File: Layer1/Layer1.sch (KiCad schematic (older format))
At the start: 48 parts, among them IC1 74HCT4060D-Q100,11, J1 Conn_02x20_Odd_Even, J2 Conn_02x20_Odd_Even, J3 Conn_02x12_Odd_Even, J4 Barrel_Jack_MountingPin, Q1 2N2222, SW1 SW_Push, SW2 SW_Push, SW3 SW_DIP_x01, U1 28C256, U10 7400, U11 NE555, U2 74LS193, U3 74461, U4 28C256, U5 74154, U6 74461, U7 28C256, U8 74HCT273, U9 28C256, X1 SG-8002DC

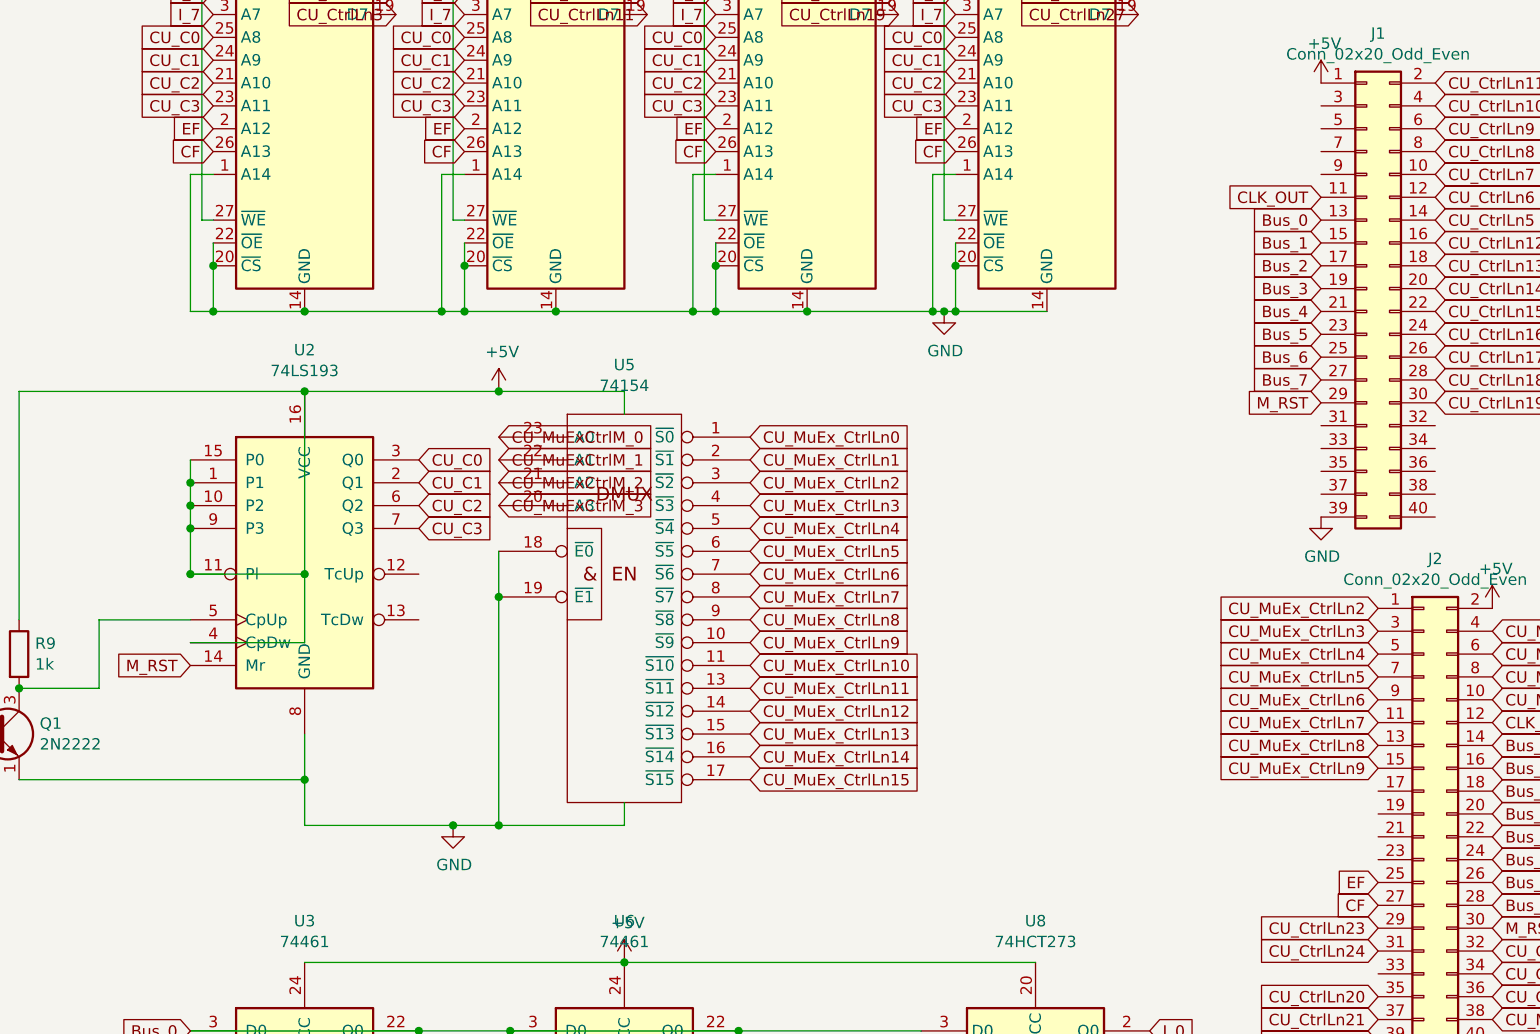
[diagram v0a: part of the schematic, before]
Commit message: Layer 3 complete
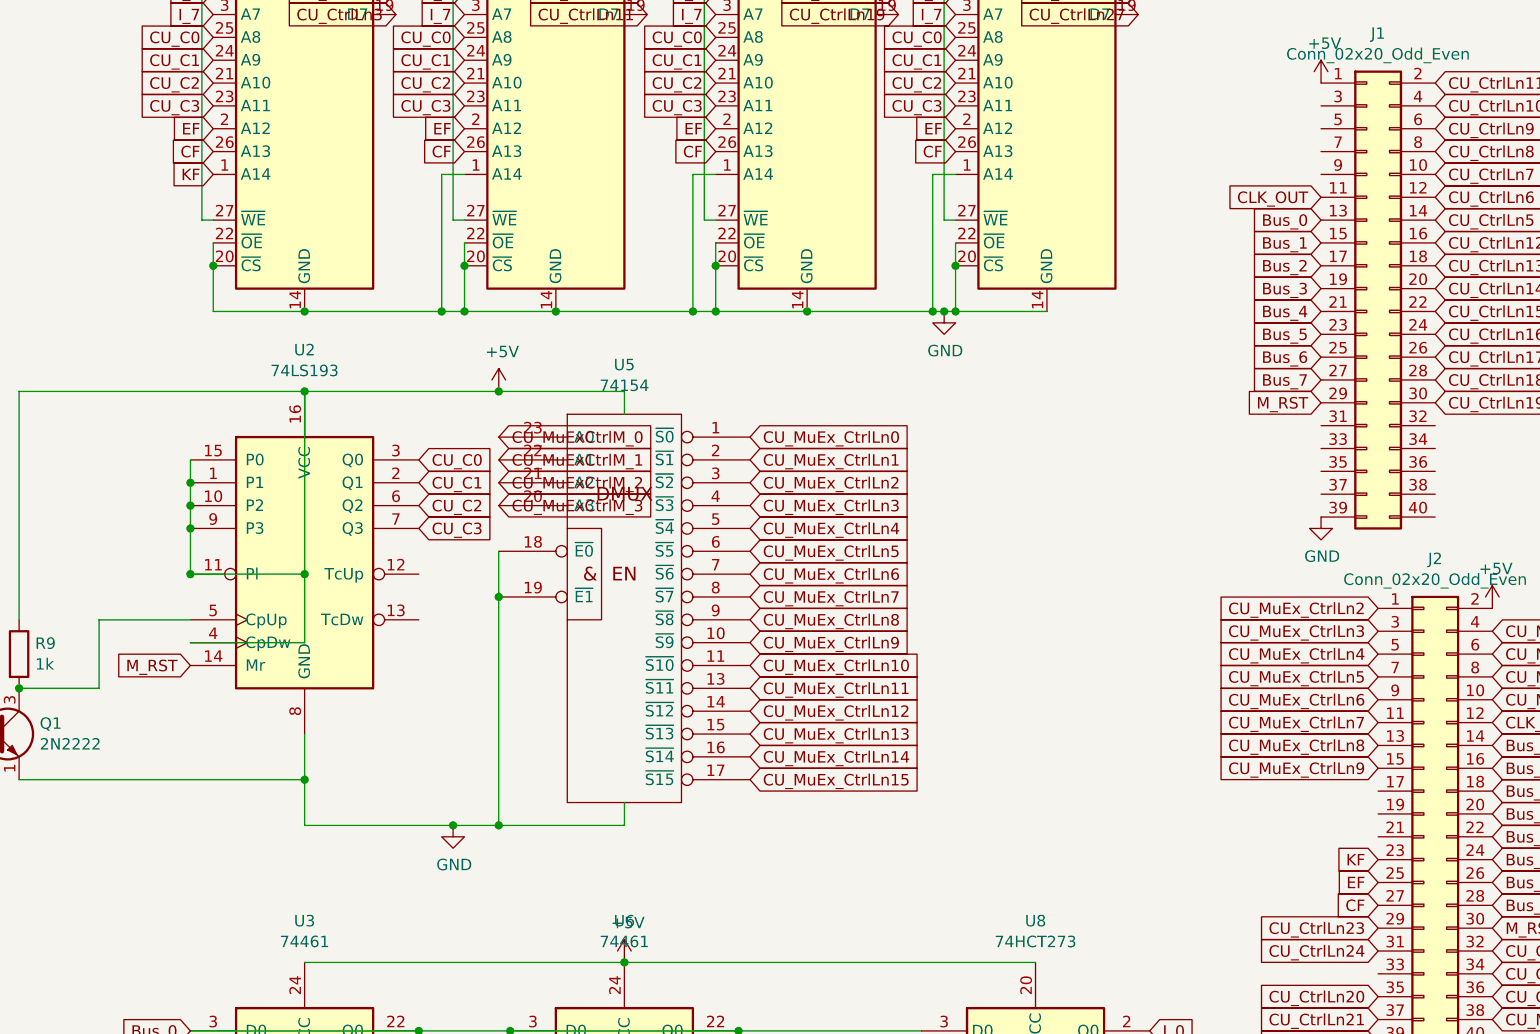
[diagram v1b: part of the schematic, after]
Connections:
- net GND: no longer U1.1 (A14)
- net KF: now reaches J2.23 (Pin_23)
- net KF: now also U1.1 (A14)
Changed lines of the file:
@@
 EESchema Schematic File Version 4
+LIBS:Layer1-cache
 EELAYER 30 0
 EELAYER END
@@
 Connection ~ 2500 2950
 Connection ~ 3600 2950
-Wire Wire Line
-	3600 2950 4150 2950
-Wire Wire Line
-	2500 2950 3100 2950
-Wire Wire Line
-	2100 2950 2000 2950
 Connection ~ 2100 2950
 Connection ~ 1400 2950
@@
 Text GLabel 4250 2250 0    50   Input ~ 0
 CF
-Wire Wire Line
-	1000 2350 900  2350
-Wire Wire Line
-	900  2350 900  2950
-Wire Wire Line
-	900  2950 1000 2950
-Connection ~ 1000 2950
-Wire Wire Line
-	2100 2350 2000 2350
-Wire Wire Line
-	2000 2350 2000 2950
-Connection ~ 2000 2950
-Wire Wire Line
-	2000 2950 1400 2950
-Wire Wire Line
-	3200 2350 3100 2350
-Wire Wire Line
-	3100 2350 3100 2950
-Connection ~ 3100 2950
-Wire Wire Line
-	3100 2950 3200 2950
-Wire Wire Line
-	4250 2350 4150 2350
-Wire Wire Line
-	4150 2350 4150 2950
-Connection ~ 4150 2950
-Wire Wire Line
-	4150 2950 4200 2950
 $Comp
 L Connector_Generic:Conn_02x20_Odd_Even J1
@@
 Text GLabel 6100 5550 0    50   Input ~ 0
 CF
+Wire Wire Line
+	1400 2950 2000 2950
+Wire Wire Line
+	2500 2950 3100 2950
+Wire Wire Line
+	3600 2950 4150 2950
+Text GLabel 1000 2350 0    50   Input ~ 0
+KF
+Text GLabel 6100 5350 0    50   Input ~ 0
+KF
+Wire Wire Line
+	2100 2350 2000 2350
+Wire Wire Line
+	2000 2350 2000 2950
+Connection ~ 2000 2950
+Wire Wire Line
+	2000 2950 2100 2950
+Wire Wire Line
+	3200 2350 3100 2350
+Wire Wire Line
+	3100 2350 3100 2950
+Connection ~ 3100 2950
+Wire Wire Line
+	3100 2950 3200 2950
+Wire Wire Line
+	4250 2350 4150 2350
+Wire Wire Line
+	4150 2350 4150 2950
+Connection ~ 4150 2950
+Wire Wire Line
+	4150 2950 4200 2950
 $EndSCHEMATC

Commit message: Backup
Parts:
- removed Q1: 2N2222, Package_TO_SOT_THT:TO-92, symbol Transistor_BJT:2N2219
- removed R8: 10k, Resistor_THT:R_Axial_DIN0309_L9.0mm_D3.2mm_P12.70mm_Horizontal, symbol Device:R
- removed R9: 1k, Resistor_THT:R_Axial_DIN0309_L9.0mm_D3.2mm_P12.70mm_Horizontal, symbol Device:R
- removed U10: 7400, Package_DIP:DIP-14_W7.62mm, symbol 74xx:7400
- added U10, U18: 74LS08, Package_DIP:DIP-14_W7.62mm_LongPads, symbol 74xx:74LS08
- added U12, U16, U20: 74LS04, Package_DIP:DIP-14_W7.62mm_LongPads, symbol 74xx:74LS04
- added U13, U15, U17: 74LS02, Package_DIP:DIP-14_W7.62mm_LongPads, symbol 74xx:74LS02
- added U14, U19: 74LS00, Package_DIP:DIP-14_W7.62mm_LongPads, symbol 74xx:74LS00
- added U21: SST39SF010, Package_DIP:DIP-32_W15.24mm_LongPads, symbol Memory_Flash:SST39SF010
- added U22: 74HC238, Package_DIP:DIP-16_W7.62mm_LongPads, symbol 74xx_IEEE:74HC238
- added U23: 74LS138, Package_DIP:DIP-16_W7.62mm_LongPads, symbol 74xx_IEEE:74LS138
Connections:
- net +5V: now also U10.14 (VCC), U12.14 (VCC), U13.14 (VCC), U14.14 (VCC), U15.14 (VCC), U16.14 (VCC), U17.14 (VCC), U19.14 (VCC), U20.14 (VCC), U21.32 (VCC), U22.16 (VCC), U23.16 (VCC), U23.6 (G1)
- net 555_OUT: now also U19.1
- net BTN_OUT: now also U19.5
- net CF: now also U21.28 (A13)
- net CLK_OUT: now also U16.11
- net CU_C0: now also J1.3 (Pin_3), U21.27 (A8)
- net CU_C1: now also J1.5 (Pin_5), U21.26 (A9)
- net CU_C2: now also J1.7 (Pin_7), U21.23 (A10)
- net CU_C3: now also J1.9 (Pin_9), U21.25 (A11)
- net CU_CtrlLn0: now also U10.12, U13.1
- net CU_CtrlLn1: now also U10.9, U14.8
- net CU_CtrlLn2: now also U10.4, U13.10
- net CU_CtrlLn27: now also U2.14 (Mr)
- net CU_CtrlLn3: now also U10.1, U14.3
- net CU_CtrlLn4: now also U15.2, U15.5, U17.3, U22.14 (Y1); no longer U8.11 (Cp)
- net CU_CtrlLn5: now also U15.3, U16.3, U17.8
- net CU_CtrlLn6: now also U15.6, U16.5
- net CU_MuEx_CtrlLn0: now also U5.3 (~S2); no longer U5.1 (~S0)
- net CU_MuEx_CtrlLn1: now also U5.4 (~S3); no longer U5.2 (~S1)
- net CU_MuEx_CtrlLn10: no longer U5.11 (~S10)
- net CU_MuEx_CtrlLn11: no longer U5.13 (~S11)
- net CU_MuEx_CtrlLn12: no longer U5.14 (~S12)
- net CU_MuEx_CtrlLn13: no longer U5.15 (~S13)
- net CU_MuEx_CtrlLn14: no longer U5.16 (~S14)
- net CU_MuEx_CtrlLn15: no longer U5.17 (~S15)
- net CU_MuEx_CtrlLn2: no longer U5.3 (~S2)
- net CU_MuEx_CtrlLn3: no longer U5.4 (~S3)
- net CU_MuEx_CtrlLn4: no longer U5.5 (~S4)
- net CU_MuEx_CtrlLn5: no longer U5.6 (~S5)
- net CU_MuEx_CtrlLn6: no longer U5.7 (~S6)
- net CU_MuEx_CtrlLn7: no longer U5.8 (~S7)
- net CU_MuEx_CtrlLn8: no longer U5.9 (~S8)
- net CU_MuEx_CtrlLn9: no longer U5.10 (~S9)
- net Debug_CLK_OUT: now also U19.8
- net EF: now also U21.4 (A12)
- net GND: now also U10.7 (GND), U12.7 (GND), U13.7 (GND), U14.7 (GND), U15.7 (GND), U16.7 (GND), U17.7 (GND), U19.7 (GND), U20.7 (GND), U21.16 (GND), U21.2 (A16), U21.22 (CE), U21.24 (OE), U22.5 (~G2B), U22.8 (GND), U23.8 (GND); no longer U4.1 (A14), U5.18 (~E0), U7.1 (A14), U9.1 (A14)
- net I_0: now also J1.31 (Pin_31), U21.12 (A0)
- net I_1: now also J1.33 (Pin_33), U21.11 (A1)
- net I_2: now also J1.35 (Pin_35), U21.10 (A2)
- net I_3: now also J1.37 (Pin_37), U21.9 (A3)
- net I_4: now also J1.32 (Pin_32), U21.8 (A4)
- net I_5: now also J1.34 (Pin_34), U21.7 (A5)
- net I_6: now also J1.36 (Pin_36), U18.12, U21.6 (A6); no longer U1.4 (A6)
- net I_7: now also J1.38 (Pin_38), U18.13, U21.5 (A7); no longer U1.3 (A7)
- net KF: now also U1.3 (A7), U21.29 (A14); no longer U1.1 (A14)
- net M_RST: now also U1.1 (A14), U4.1 (A14), U7.1 (A14), U9.1 (A14), U21.3 (A15); no longer U2.14 (Mr)
- net Switch_OUT: now also U16.9, U19.4
- net at U2.5 (CpUp): now also U16.10
- net CU_CtrlLn7 renamed ALU_M
- net CU_MuExCtrlM_0 renamed CU_MuExCtrlOut_0
- net CU_MuExCtrlOut_0: now also U21.13 (D0)
- net CU_MuExCtrlM_1 renamed CU_MuExCtrlOut_1
- net CU_MuExCtrlOut_1: now also U21.14 (D1)
- net CU_MuExCtrlM_2 renamed CU_MuExCtrlOut_2
- net CU_MuExCtrlOut_2: now also U21.15 (D2)
- net CU_MuExCtrlM_3 renamed CU_MuExCtrlOut_3
- net CU_MuExCtrlOut_3: now also U21.17 (D3)
- new net: U1.4 (A6), U18.11
- new net: U18.4, U5.7 (~S6)
- new net: U16.8, U19.2
- new net: U10.6, U12.2, U13.2, U13.3, U13.5, U13.8, U14.12, U14.2, U15.11, U18.1
- new net: U10.8, U13.11, U13.9, U14.10, U14.4, U15.9, U18.2
- new net: U10.11, U12.13, U14.13, U14.5, U18.10
- new net: U12.3, U18.8
- new net: U10.3, U12.1, U14.1, U14.9, U18.9
- new net: U16.4, U17.12
- new net: U16.6, U17.6, U17.9
- new net: U12.12, U13.12, U13.6
- new net: U15.4, U17.11
- new net: U17.10, U17.2
- new net: U16.13, U17.4
- new net: U12.4, U15.12, U15.8
- new net: U19.3, U19.9
- new net: U19.10, U19.6
- new net: U19.12, U23.12 (~Y3)
- new net ALU_Out: U19.13, U23.11 (~Y4), U5.18 (~E0)
- new net ALU_S0-Cn: U16.12
- new net ALU_S1: U17.1
- new net ALU_S2: U17.13
- new net ALU_S3: U15.1, U17.5
- new net A_In: U19.11
- new net A_Out: U5.5 (~S4)
- new net B_In: U22.13 (Y2)
- new net B_Out: U5.6 (~S5)
- new net Bank_Reg_In: U23.13 (~Y2)
- new net CU_MuExCtrlIn_0: U21.18 (D4), U22.1 (A0), U23.1 (A0)
- new net CU_MuExCtrlIn_1: U21.19 (D5), U22.2 (A1), U23.2 (A1)
- new net CU_MuExCtrlIn_2: U21.20 (D6), U22.3 (A2), U23.3 (A2)
- new net CU_MuExCtrlIn_3: U21.21 (D7), U22.6 (G1), U23.5 (~G2B)
- new net C_In: U22.12 (Y3)
- new net C_Out: U18.6
- new net Counter_Control: U16.1, U18.5, U5.13 (~S11)
- new net Counter_Countrol_Inverted: U10.10, U10.13, U10.2, U10.5, U16.2, U22.4 (~G2A), U23.4 (~G2A)
- new net D_In: U22.11 (Y4)
- new net D_Out: U5.8 (~S7)
- new net Mem_Add_H_In: U22.9 (Y6)
- new net Mem_Add_L_In: U22.10 (Y5)
- new net PS2_Out: U5.11 (~S10)
- new net Ram_In: U23.15 (~Y0)
- new net Ram_Out: U5.9 (~S8)
- new net SP_Clr: U18.3
- new net SP_Down: U15.13
- new net SP_OE: U5.2 (~S1)
- new net SP_Up: U15.10
- new net VM_H_CTRL0: U13.13
- new net VM_H_CTRL1: U14.11
- new net VM_L_CTRL0: U13.4
- new net VM_L_CTRL1: U14.6
- new net VRam_OE: U5.10 (~S9)
- new net VRam_WE: U23.14 (~Y1)
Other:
- moved on the sheet: U2, U5
